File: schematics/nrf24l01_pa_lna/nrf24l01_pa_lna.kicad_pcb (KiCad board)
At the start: 4 copper layers, 43.5 x 13.5 mm, 46 parts, among them J1 Conn_Coaxial_Small, J3 Conn_02x04_Odd_Even, U1 NRF24L01, U3 MCP1802x-xx02xOT, Y1 Crystal

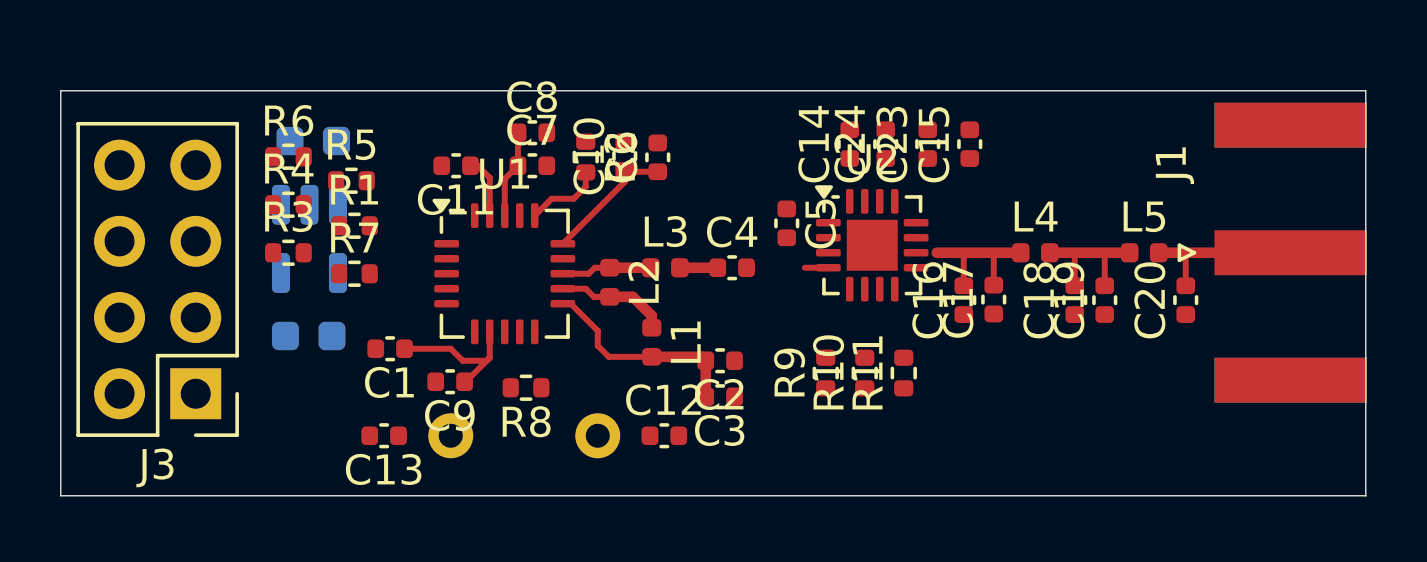
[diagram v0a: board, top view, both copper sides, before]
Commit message: a
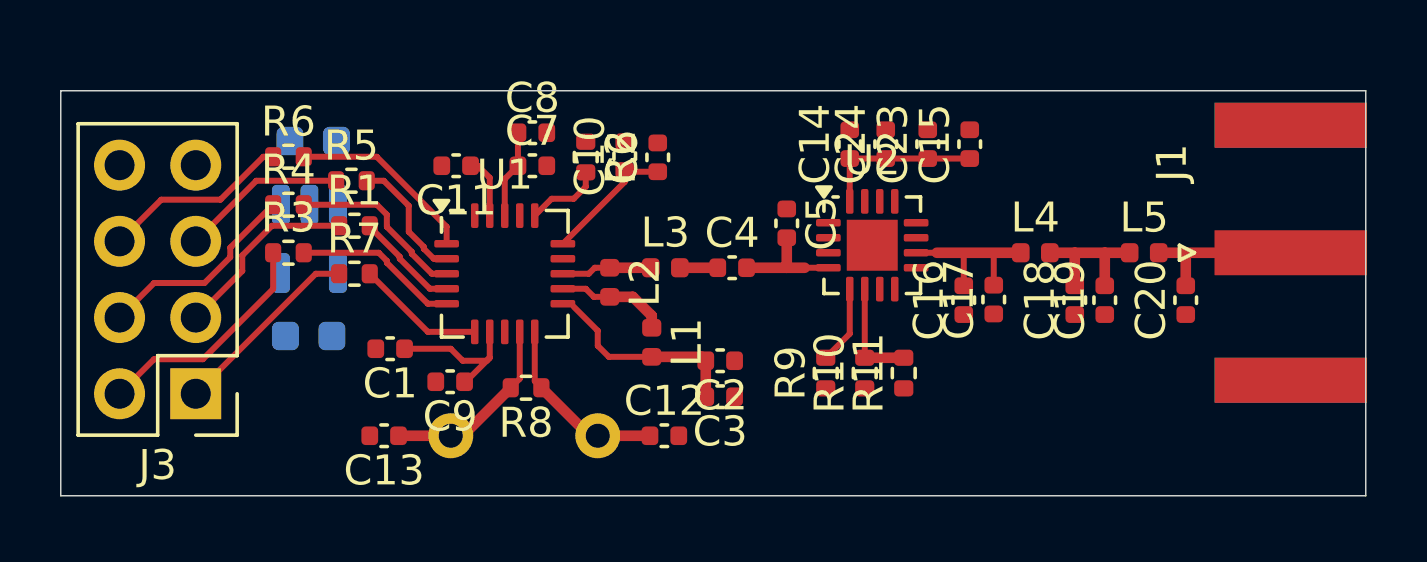
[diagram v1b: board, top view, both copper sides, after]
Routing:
- net /miso: track 0.00 -> 7.77 mm
- net /sck: track 0.00 -> 6.86 mm
- net /irq: track 0.00 -> 6.44 mm
- net /xc2: track 0.00 -> 6.39 mm
- net /mosi: track 0.00 -> 6.35 mm
- net Net-(U1-CE): track 0.00 -> 6.30 mm
- net /ce: track 0.00 -> 6.29 mm
- net /xc1: track 0.00 -> 6.24 mm
- net Net-(U1-SCK): track 0.00 -> 5.99 mm
- net /scn: track 0.00 -> 5.52 mm
- net Net-(U1-MISO): track 0.00 -> 5.50 mm
- net VDD: track 12.4 -> 17.9 mm
- net Net-(U1-IRQ): track 0.00 -> 4.30 mm
- net Net-(U1-CSN): track 0.00 -> 4.28 mm
- net Net-(U2-rxen): track 0.00 -> 3.59 mm
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
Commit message: Finished the design in bulk...
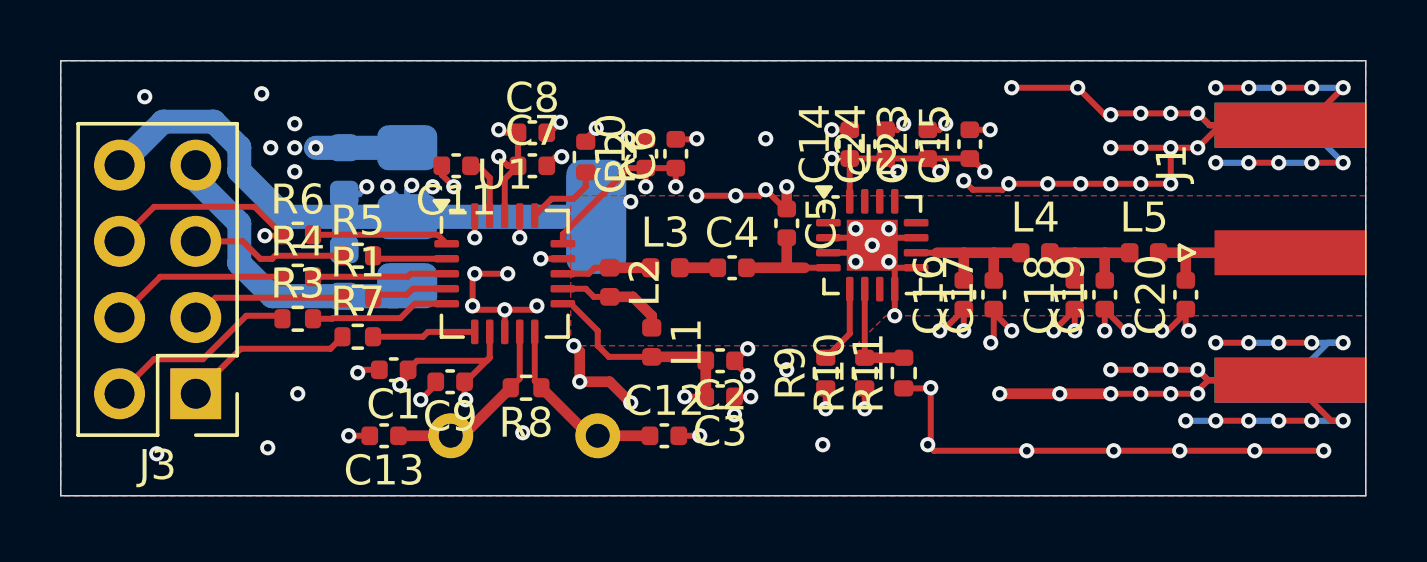
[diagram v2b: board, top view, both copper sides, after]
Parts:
- removed U3: MCP1802x-xx02xOT, Package_TO_SOT_SMD:SOT-23-5
- added U4: MCP1825S, Package_TO_SOT_SMD:SOT-223-3_TabPin2, B.Cu at (133.7, 94.7)
- moved C22 5.63 mm to (128.4, 93.2), turned to -90 degrees
- moved C21 4.52 mm to (128.4, 96.6), turned to 90 degrees
- moved R6 2.62 mm to (126.9, 95.3)
- moved R5 2.51 mm to (128.9, 96.0)
- moved R4 2.42 mm to (126.9, 96.7)
- moved R1 2.40 mm to (128.9, 97.4)
- moved R3 2.22 mm to (126.9, 98.1)
- moved R7 2.10 mm to (128.9, 98.7)
- moved C1 0.71 mm to (130.1, 99.8)
- moved C10 0.70 mm to (138.5, 92.6)
- moved C6 0.61 mm to (139.5, 92.6)
- moved C16 0.18 mm to (149.1, 97.3)
- moved C18 0.18 mm to (152.8, 97.3)
- moved C19 0.18 mm to (153.8, 97.3)
- moved C20 0.18 mm to (156.5, 97.3)
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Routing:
- net GND: track 0.00 -> 277.7 mm, vias 0 -> 118
- net VDD: track 17.9 -> 91.5 mm, vias 0 -> 15
- net /ce: track 6.29 -> 35.7 mm, vias 0 -> 2
- net /v_pwr: track 0.00 -> 10.1 mm
- net /vdd_pa: track 6.64 -> 13.7 mm, vias 0 -> 2
- net Net-(U1-CSN): track 4.28 -> 2.49 mm
- net Net-(U1-CE): track 6.30 -> 4.58 mm
- net Net-(U1-SCK): track 5.99 -> 4.49 mm
- net /miso: track 7.77 -> 6.55 mm
- net /mosi: track 6.35 -> 5.16 mm
- net Net-(U1-MOSI): track 3.49 -> 2.58 mm
- net /sck: track 6.86 -> 5.99 mm
- net Net-(U1-IRQ): track 4.30 -> 3.46 mm
- net Net-(U1-MISO): track 5.50 -> 4.66 mm
- net /irq: track 6.44 -> 5.68 mm
- added copper zone on B.Cu, net GND
- added copper zone on F.Cu, net GND
- added copper zone on In1.Cu, net GND
- added copper zone on In2.Cu, net GND
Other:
- board size 43.5 x 13.5 mm -> 43.5 x 14.5 mm
